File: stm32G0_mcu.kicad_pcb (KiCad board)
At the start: 4 copper layers, 75 x 40 mm, 44 parts, among them J1 Conn_01x04_Pin, J2 Conn_01x06_Pin, J3 Conn_01x04_Pin, SW1 SW_Nidec_CAS-120A1, SW2 SW_Push, U1 STM32G0B0KETx, U7 MCP2200-I-SO, X1 12M

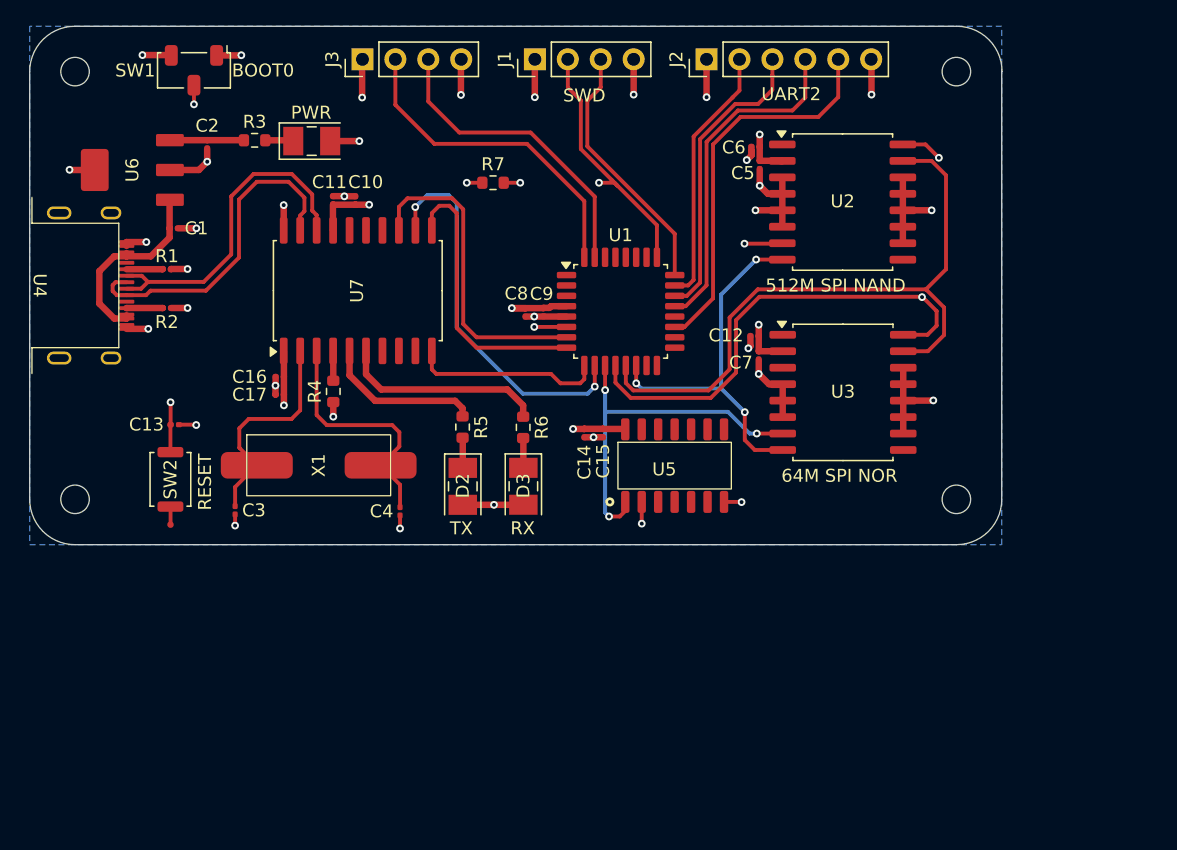
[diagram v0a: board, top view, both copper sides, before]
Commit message: asdfsa
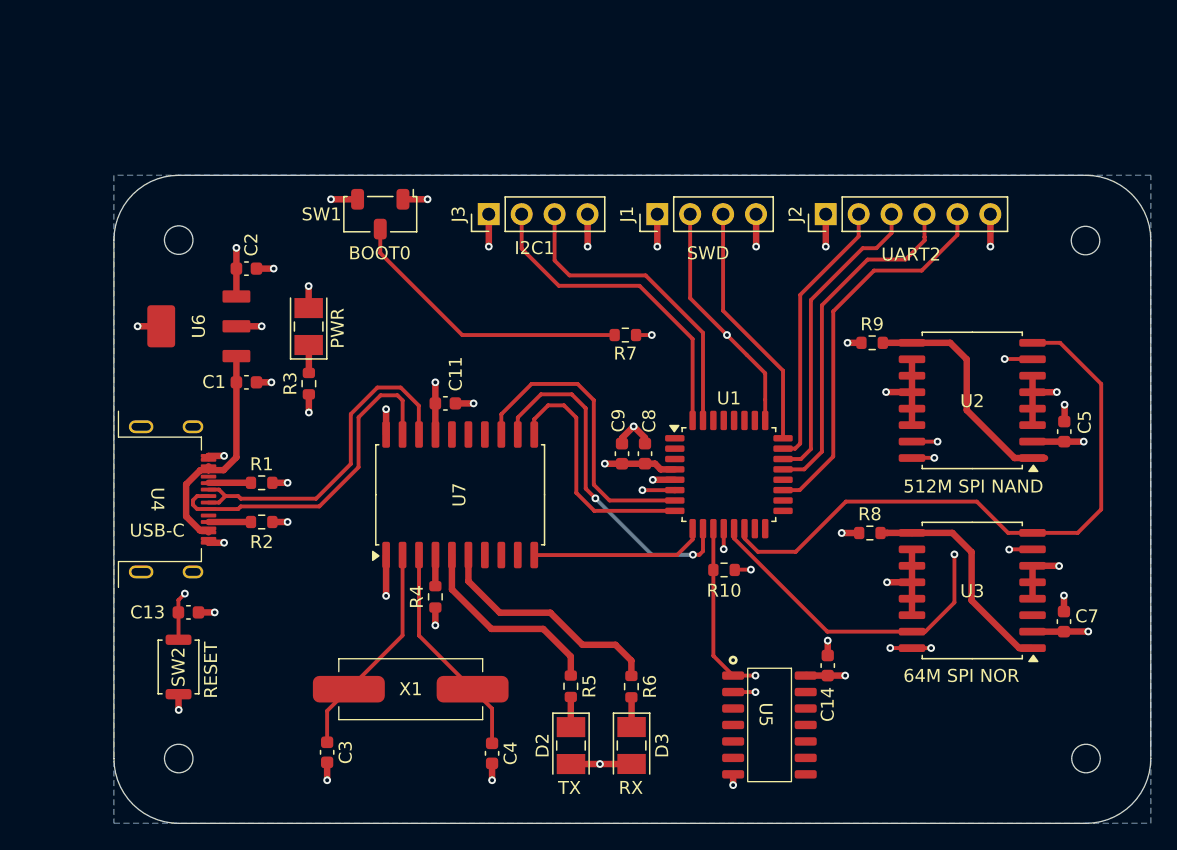
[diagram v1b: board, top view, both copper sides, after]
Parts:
- removed C10, C12, C16, C17, C6: C, Capacitor_SMD:C_0201_0603Metric
- removed C15: 100u, Capacitor_SMD:C_0201_0603Metric
- added R10: 10k, Resistor_SMD:R_0603_1608Metric, F.Cu at (137.1, 110.5)
- added R8: 10k, Resistor_SMD:R_0603_1608Metric, F.Cu at (148.3, 107.6)
- added R9: 10k, Resistor_SMD:R_0603_1608Metric, F.Cu at (148.5, 92.9)
- C1, C11, C13, C14, C2, C3, C4, C8, C9: footprint Capacitor_SMD:C_0201_0603Metric -> Capacitor_SMD:C_0603_1608Metric
- C5, C7: value C -> 220n; footprint Capacitor_SMD:C_0201_0603Metric -> Capacitor_SMD:C_0603_1608Metric
- R1, R2: footprint Resistor_SMD:R_0201_0603Metric -> Resistor_SMD:R_0603_1608Metric
- moved C7 31.2 mm to (163.3, 114.4), turned to 90 degrees
- moved C5 31.2 mm to (163.3, 99.8), turned to 90 degrees
- moved C14 26.0 mm to (145.1, 117.8), turned to 90 degrees
- moved H3 22.4 mm to (165.0, 125.0)
- moved R6 21.7 mm to (129.9, 119.5)
- moved D2 21.7 mm to (125.3, 124.0)
- moved D3 21.7 mm to (129.9, 124.0)
- moved R5 21.7 mm to (125.2, 119.4)
- moved H4 21.5 mm to (95.0, 125.0)
- moved U5 21.3 mm to (140.6, 122.4), turned to -90 degrees
- moved C3 20.0 mm to (106.5, 124.5)
- moved C4 20.0 mm to (119.2, 124.6)
- moved R3 19.2 mm to (105.0, 96.1), turned to 90 degrees
- moved U4 19.1 mm to (93.3, 105.0)
- moved X1 18.7 mm to (112.9, 119.7)
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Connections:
- net Net-(D1-A) renamed /POWER_SUPPLY/PWR_LED
- net UART_RX renamed UART2_RX
- C1 pad 1: Net-(U6-IN) -> +5V_USB
- C3 pad 1: OSC -> /UART/OSC1
- C4 pad 1: OSC -> /UART/OSC2
- D2 pad 2: TxLED -> Net-(D2-A)
- D3 pad 2: RxLED -> Net-(D3-A)
- R1 pad 1: Net-(U4-CC1) -> /POWER_SUPPLY/CC
- R2 pad 1: Net-(U4-CC2) -> /POWER_SUPPLY/CC
- R5 pad 1: TxLED -> /UART/TX_LED
- R5 pad 2: TxLED -> Net-(D2-A)
- R6 pad 1: RxLED -> /UART/RX_LED
- R6 pad 2: RxLED -> Net-(D3-A)
- R7 pad 1: Net-(SW1-B) -> BOOT0
- SW1 pad 2: Net-(SW1-B) -> BOOT0
- U2 pad 1: unconnected-(U2-HOLD(IO_{3})-Pad1) -> Net-(U2-HOLD(IO_{3}))
- U2 pad 15: /FLASH/SPI10 -> SPI1_MOSI
- U2 pad 7: FLASH_NAND_CS -> FLASH_CS
- U2 pad 8: /FLASH/SPI11 -> SPI1_MISO
- U2 pad 9: unconnected-(U2-WP(IO_{2})-Pad9) -> Net-(U2-HOLD(IO_{3}))
- U3 pad 1: unconnected-(U3-HOLD(IO_{3})-Pad1) -> Net-(U3-HOLD(IO_{3}))
- U3 pad 15: /FLASH/SPI10 -> SPI1_MOSI
- U3 pad 7: FLASH_CS -> FLASH_NOR_CS
- U3 pad 8: /FLASH/SPI11 -> SPI1_MISO
- U3 pad 9: unconnected-(U3-WP(IO_{2})-Pad9) -> Net-(U3-HOLD(IO_{3}))
- U4 pad A5: Net-(U4-CC1) -> /POWER_SUPPLY/CC
- U4 pad B5: Net-(U4-CC2) -> /POWER_SUPPLY/CC
- U5 pad 2: FLASH_NAND_CS -> FLASH_NOR_CS
- U6 pad 1: Net-(U6-IN) -> +5V_USB
- U7 pad 10: UART_TX -> UART2_TX
- U7 pad 11: UART_RTS -> UART2_RTS
- U7 pad 13: UART_CTS -> UART2_CTS
- U7 pad 2: OSC -> /UART/OSC1
- U7 pad 3: OSC -> /UART/OSC2
- U7 pad 5: TxLED -> /UART/TX_LED
- U7 pad 6: RxLED -> /UART/RX_LED
- X1 pad 1: OSC -> /UART/OSC1
- X1 pad 2: OSC -> /UART/OSC2
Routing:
- net OSC: track 36.0 -> 0.00 mm
- net FLASH_NAND_CS: track 33.0 -> 0.00 mm, vias 2 -> 0
- net FLASH_NOR_CS: track 0.00 -> 31.6 mm, vias 0 -> 2
- net FLASH_CS: track 28.3 -> 57.9 mm, vias 3 -> 2
- net Net-(SW1-B): track 26.2 -> 0.00 mm, vias 2 -> 0
- net UART_CTS: track 24.6 -> 0.00 mm
- net UART2_CTS: track 0.00 -> 23.5 mm
- net UART_RTS: track 21.7 -> 0.00 mm
- net BOOT0: track 27.0 -> 47.9 mm
- net UART2_RTS: track 0.00 -> 19.2 mm
- net SPI1_MISO: track 29.2 -> 48.4 mm, vias 3 -> 0
- net Net-(U2-HOLD(IO_{3})): track 0.00 -> 18.5 mm
- net /UART/RX_LED: track 0.00 -> 18.3 mm
- net RxLED: track 18.1 -> 0.00 mm
- net Net-(U3-HOLD(IO_{3})): track 0.00 -> 17.6 mm
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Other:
- board size 75 x 40 mm -> 80 x 50 mm
- board text added: "I2C1"
- board text added: "KabelitzJ STM32G0 Dev Board Rev 1 29.10.2024"
